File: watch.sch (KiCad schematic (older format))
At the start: 22 parts, among them P1 CONN_6, SW1 SW_PUSH, SW2 SW_PUSH, SW3 SW_PUSH, SW4 SW_PUSH, U1 nrf51822, U3 S25FL1-K, X1 16MHz, X2 32.768kHz

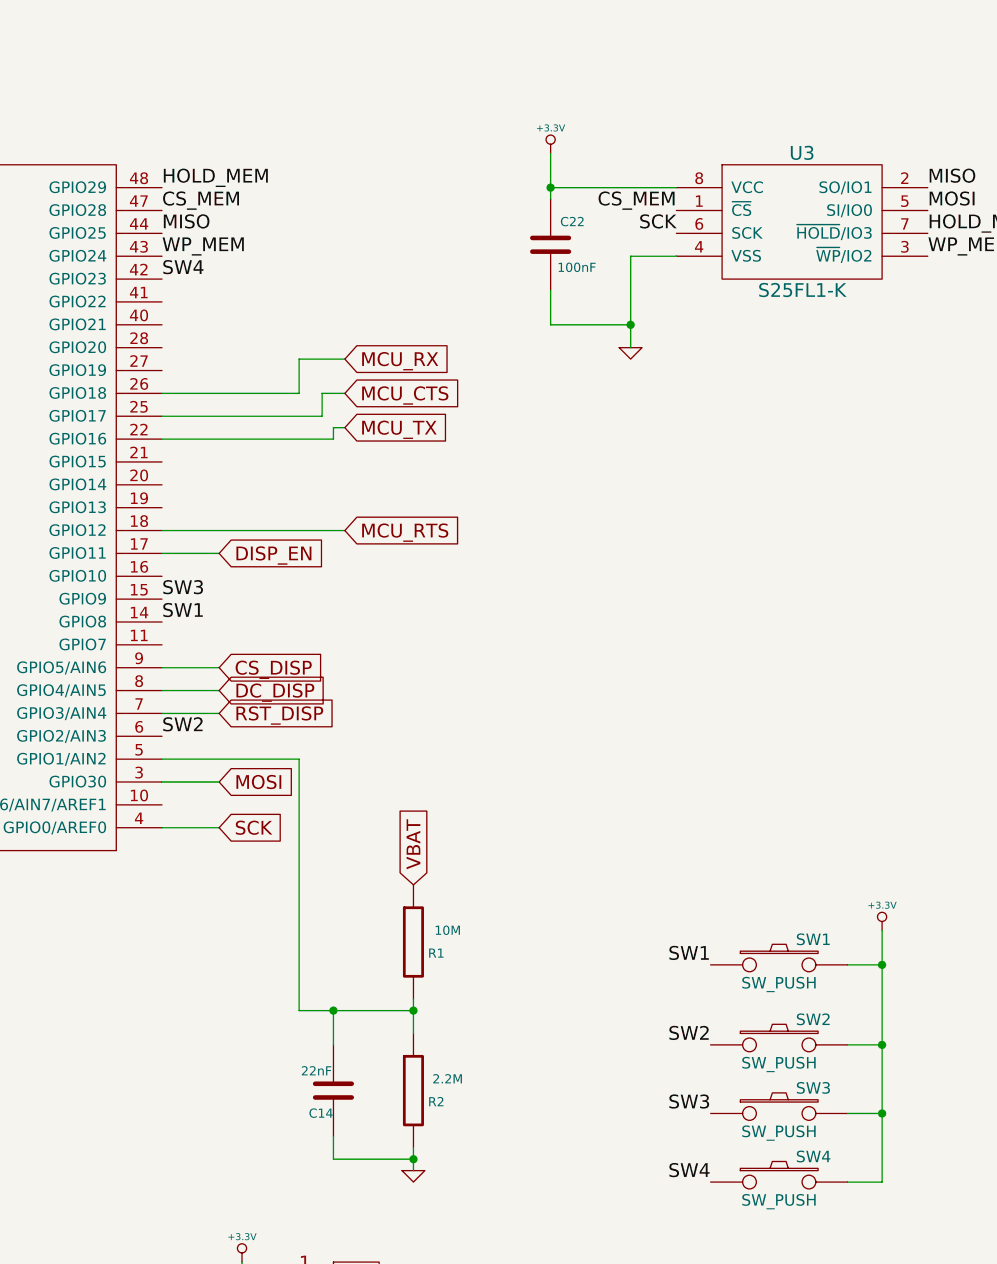
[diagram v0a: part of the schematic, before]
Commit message: Added .gitignore, finished midmount layout
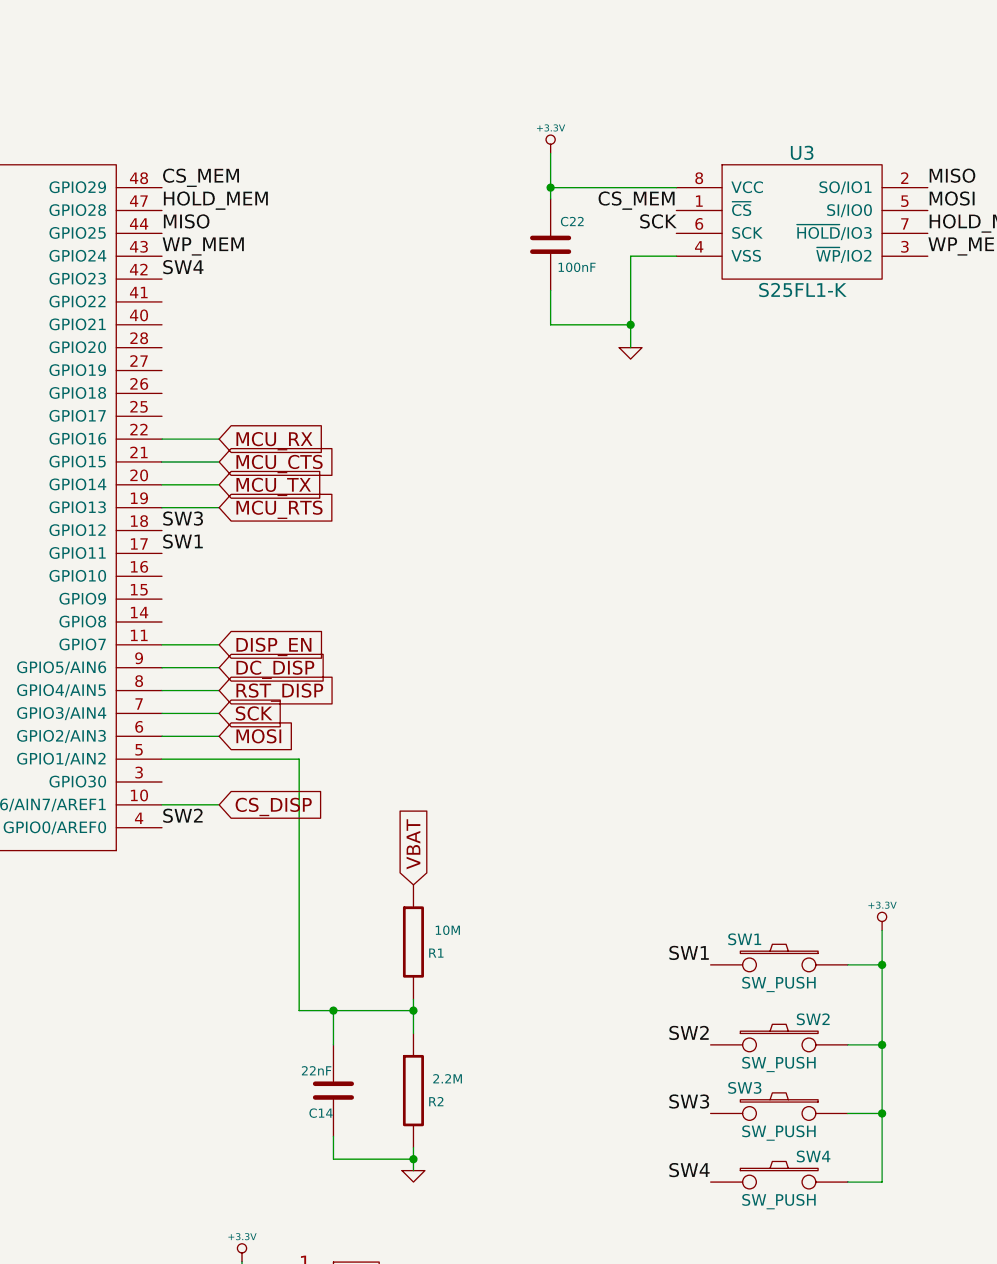
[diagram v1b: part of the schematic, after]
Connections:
- net +3.3V: now also SW1.1, SW3.1; no longer SW1.2, SW3.2
- net CS_DISP: now also U1.10 (GPIO6/AIN7/AREF1); no longer U1.9 (GPIO5/AIN6)
- net CS_MEM: now also U1.48 (GPIO29); no longer U1.47 (GPIO28)
- net DC_DISP: now also U1.9 (GPIO5/AIN6); no longer U1.8 (GPIO4/AIN5)
- net DISP_EN: now also U1.11 (GPIO7); no longer U1.17 (GPIO11)
- net HOLD_MEM: now also U1.47 (GPIO28); no longer U1.48 (GPIO29)
- net MCU_CTS: now also U1.21 (GPIO15); no longer U1.25 (GPIO17)
- net MCU_RTS: now also U1.19 (GPIO13); no longer U1.18 (GPIO12)
- net MCU_RX: now also U1.22 (GPIO16); no longer U1.26 (GPIO18)
- net MCU_TX: now also U1.20 (GPIO14); no longer U1.22 (GPIO16)
- net MOSI: now also U1.6 (GPIO2/AIN3); no longer U1.3 (GPIO30)
- net RST_DISP: now also U1.8 (GPIO4/AIN5); no longer U1.7 (GPIO3/AIN4)
- net SCK: now also U1.7 (GPIO3/AIN4); no longer U1.4 (GPIO0/AREF0)
- net SW1: now also SW1.2, U1.17 (GPIO11); no longer SW1.1, U1.14 (GPIO8)
- net SW2: now also U1.4 (GPIO0/AREF0); no longer U1.6 (GPIO2/AIN3)
- net SW3: now also SW3.2, U1.18 (GPIO12); no longer SW3.1, U1.15 (GPIO9)
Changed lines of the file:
@@
 Text Label 5900 1950 0    60   ~ 0
 MISO
-Text Label 5900 1850 0    60   ~ 0
+Text Label 5900 1750 0    60   ~ 0
 CS_MEM
 Text Label 8150 1850 2    60   ~ 0
@@
 Text Label 9250 1750 0    60   ~ 0
 MISO
-Text Label 5900 1750 0    60   ~ 0
+Text Label 5900 1850 0    60   ~ 0
 HOLD_MEM
 Text Label 9250 1950 0    60   ~ 0
@@
 F 3 "" H 8600 5150 60  0000 C CNN
 	1    8600 5150
-	1    0    0    -1
+	-1   0    0    -1
 $EndComp
 $Comp
@@
 F 3 "" H 8600 5800 60  0000 C CNN
 	1    8600 5800
-	1    0    0    -1
+	-1   0    0    -1
 $EndComp
 $Comp
@@
 Text Label 8300 6100 2    60   ~ 0
 SW4
-Text Label 5900 3650 0    60   ~ 0
+Text Label 5900 3350 0    60   ~ 0
 SW1
-Text Label 5900 4150 0    60   ~ 0
+Text Label 5900 4550 0    60   ~ 0
 SW2
-Text Label 5900 3550 0    60   ~ 0
+Text Label 5900 3250 0    60   ~ 0
 SW3
 Text Label 5900 2150 0    60   ~ 0
@@
 Wire Wire Line
 	6500 5350 6500 4250
-Wire Wire Line
-	6500 4250 5900 4250
 Connection ~ 7000 5350
 $Comp
@@
 Wire Wire Line
 	6000 6900 6000 7200
-Text GLabel 6700 2650 2    60   Input ~ 0
+Text GLabel 6150 2950 2    60   Input ~ 0
 MCU_CTS
-Text GLabel 6700 3250 2    60   Input ~ 0
+Text GLabel 6150 3150 2    60   Input ~ 0
 MCU_RTS
-Text GLabel 6700 2800 2    60   Input ~ 0
+Text GLabel 6150 3050 2    60   Input ~ 0
 MCU_TX
-Text GLabel 6700 2500 2    60   Input ~ 0
+Text GLabel 6150 2850 2    60   Input ~ 0
 MCU_RX
 $Sheet
@@
 	1    0    0    -1
 $EndComp
+Text GLabel 6150 3850 2    60   Input ~ 0
+DC_DISP
 Text GLabel 6150 3950 2    60   Input ~ 0
-DC_DISP
+RST_DISP
+Text GLabel 6150 4450 2    60   Input ~ 0
+CS_DISP
+Wire Wire Line
+	6150 3950 5900 3950
+Wire Wire Line
+	5900 3850 6150 3850
 Text GLabel 6150 4050 2    60   Input ~ 0
-RST_DISP
-Text GLabel 6150 3850 2    60   Input ~ 0
-CS_DISP
+SCK
+Text GLabel 6150 4150 2    60   Input ~ 0
+MOSI
 Wire Wire Line
 	6150 4050 5900 4050
 Wire Wire Line
-	5900 3950 6150 3950
-Text GLabel 6150 4550 2    60   Input ~ 0
-SCK
-Text GLabel 6150 4350 2    60   Input ~ 0
-MOSI
-Wire Wire Line
-	6150 4550 5900 4550
-Wire Wire Line
-	6150 4350 5900 4350
-Text GLabel 6150 3350 2    60   Input ~ 0
+	6150 4150 5900 4150
+Text GLabel 6150 3750 2    60   Input ~ 0
 DISP_EN
-Wire Wire Line
-	6600 2750 5900 2750
-Wire Wire Line
-	6700 2650 6600 2650
-Wire Wire Line
-	6600 2650 6600 2750
-Wire Wire Line
-	6700 2500 6500 2500
-Wire Wire Line
-	6500 2500 6500 2650
-Wire Wire Line
-	6500 2650 5900 2650
-Wire Wire Line
-	5900 2850 6650 2850
-Wire Wire Line
-	6650 2850 6650 2800
-Wire Wire Line
-	6650 2800 6700 2800
-Wire Wire Line
-	6700 3250 5900 3250
 Text Label 5900 2050 0    60   ~ 0
 WP_MEM
 Wire Wire Line
-	6150 3850 5900 3850
-Wire Wire Line
-	5900 3350 6150 3350
+	6150 4450 5900 4450
+Wire Wire Line
+	5900 3750 6150 3750
 $Comp
 L GND #PWR015
@@
 	7600 2350 7950 2350
 Connection ~ 7950 2350
+Wire Wire Line
+	5900 2850 6150 2850
+Wire Wire Line
+	6150 3150 5900 3150
+Wire Wire Line
+	5900 3050 6150 3050
+Wire Wire Line
+	6150 2950 5900 2950
+Wire Wire Line
+	6500 4250 5900 4250
 $EndSCHEMATC
